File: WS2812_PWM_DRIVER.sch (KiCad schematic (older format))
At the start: 1 part

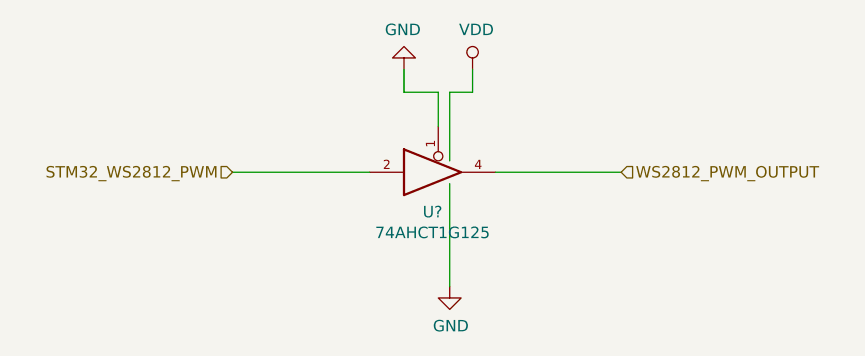
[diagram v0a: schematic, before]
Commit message: update,
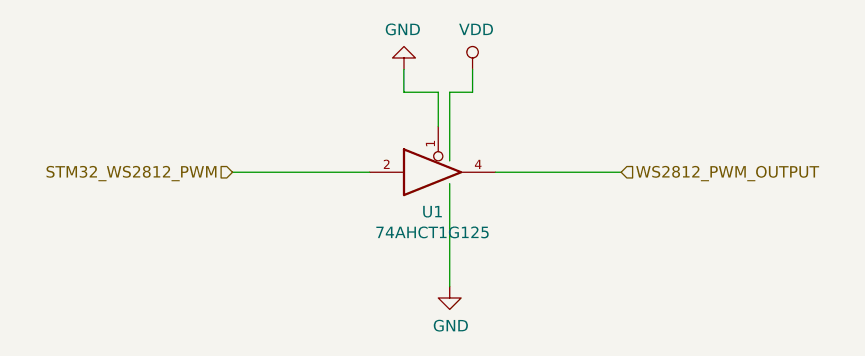
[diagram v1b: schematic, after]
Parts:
- gave numbers to parts that had none: 1
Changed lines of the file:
@@
 EESchema Schematic File Version 4
+LIBS:stm32_bottom_board_respin-cache
 EELAYER 26 0
 EELAYER END
 $Descr A4 11693 8268
 encoding utf-8
-Sheet 2 3
+Sheet 2 6
 Title ""
 Date ""
@@
 $EndDescr
 $Comp
-L 74xGxx:74AHCT1G125 U?
+L 74xGxx:74AHCT1G125 U1
 U 1 1 5BCB46C2
 P 5400 3200
-F 0 "U?" H 5375 3026 50  0000 C CNN
+F 0 "U1" H 5375 3026 50  0000 C CNN
 F 1 "74AHCT1G125" H 5375 2935 50  0000 C CNN
 F 2 "" H 5400 3200 50  0001 C CNN
@@
 	4500 3200 5100 3200
 $Comp
-L power:VDD #PWR?
+L power:VDD #PWR0103
 U 1 1 5BCB476F
 P 5550 2750
-F 0 "#PWR?" H 5550 2600 50  0001 C CNN
+F 0 "#PWR0103" H 5550 2600 50  0001 C CNN
 F 1 "VDD" H 5567 2923 50  0000 C CNN
 F 2 "" H 5550 2750 50  0001 C CNN
@@
 $EndComp
 $Comp
-L power:GND #PWR?
+L power:GND #PWR0104
 U 1 1 5BCB47D3
 P 5250 2750
-F 0 "#PWR?" H 5250 2500 50  0001 C CNN
+F 0 "#PWR0104" H 5250 2500 50  0001 C CNN
 F 1 "GND" H 5255 2577 50  0000 C CNN
 F 2 "" H 5250 2750 50  0001 C CNN
@@
 	5450 2850 5450 3150
 $Comp
-L power:GND #PWR?
+L power:GND #PWR0105
 U 1 1 5BCB4815
 P 5450 3700
-F 0 "#PWR?" H 5450 3450 50  0001 C CNN
+F 0 "#PWR0105" H 5450 3450 50  0001 C CNN
 F 1 "GND" H 5455 3527 50  0000 C CNN
 F 2 "" H 5450 3700 50  0001 C CNN

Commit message: update,
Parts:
- U1: footprint (none) -> Package_TO_SOT_SMD:SOT-23-5_HandSoldering; symbol 74xGxx:74AHCT1G125 -> taobao-components:74AHCT1G125
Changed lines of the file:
@@
 $EndDescr
 $Comp
-L 74xGxx:74AHCT1G125 U1
+L taobao-components:74AHCT1G125 U1
 U 1 1 5BCB46C2
 P 5400 3200
 F 0 "U1" H 5375 3026 50  0000 C CNN
 F 1 "74AHCT1G125" H 5375 2935 50  0000 C CNN
-F 2 "" H 5400 3200 50  0001 C CNN
+F 2 "Package_TO_SOT_SMD:SOT-23-5_HandSoldering" H 5400 3200 50  0001 C CNN
 F 3 "http://www.ti.com/lit/sg/scyt129e/scyt129e.pdf" H 5400 3200 50  0001 C CNN
 	1    5400 3200
@@
 	4500 3200 5100 3200
 $Comp
-L power:VDD #PWR0103
+L power:VDD #PWR010
 U 1 1 5BCB476F
 P 5550 2750
-F 0 "#PWR0103" H 5550 2600 50  0001 C CNN
+F 0 "#PWR010" H 5550 2600 50  0001 C CNN
 F 1 "VDD" H 5567 2923 50  0000 C CNN
 F 2 "" H 5550 2750 50  0001 C CNN
@@
 $EndComp
 $Comp
-L power:GND #PWR0104
+L power:GND #PWR08
 U 1 1 5BCB47D3
 P 5250 2750
-F 0 "#PWR0104" H 5250 2500 50  0001 C CNN
+F 0 "#PWR08" H 5250 2500 50  0001 C CNN
 F 1 "GND" H 5255 2577 50  0000 C CNN
 F 2 "" H 5250 2750 50  0001 C CNN
@@
 	5450 2850 5450 3150
 $Comp
-L power:GND #PWR0105
+L power:GND #PWR09
 U 1 1 5BCB4815
 P 5450 3700
-F 0 "#PWR0105" H 5450 3450 50  0001 C CNN
+F 0 "#PWR09" H 5450 3450 50  0001 C CNN
 F 1 "GND" H 5455 3527 50  0000 C CNN
 F 2 "" H 5450 3700 50  0001 C CNN

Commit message: update,
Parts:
- U1: symbol taobao-components:74AHCT1G125 -> stm32_bottom_board_respin-rescue:74AHCT1G125-taobao-components
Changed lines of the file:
@@
 $EndDescr
 $Comp
-L taobao-components:74AHCT1G125 U1
+L stm32_bottom_board_respin-rescue:74AHCT1G125-taobao-components U1
 U 1 1 5BCB46C2
 P 5400 3200

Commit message: update,
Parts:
- U1: symbol stm32_bottom_board_respin-rescue:74AHCT1G125-taobao-components -> taobao-components:74AHCT1G125
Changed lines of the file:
@@
 $Descr A4 11693 8268
 encoding utf-8
-Sheet 2 6
+Sheet 6 6
 Title ""
 Date ""
@@
 $EndDescr
 $Comp
-L stm32_bottom_board_respin-rescue:74AHCT1G125-taobao-components U1
+L taobao-components:74AHCT1G125 U1
 U 1 1 5BCB46C2
 P 5400 3200
